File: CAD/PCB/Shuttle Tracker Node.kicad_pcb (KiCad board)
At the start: 2 copper layers, 98.9 x 44.1 mm, 27 parts, among them J1 Conn_01x01, J2 Conn_01x01, J3 Conn_01x01, J4 Conn_01x01, J5 Conn_01x01, J6 Conn_01x01, J7 Conn_01x01, SW1 SW_Push, SW10 SW_Push, SW11 SW_Push, SW12 SW_Push, SW13 PEC11-4215F-S24, SW2 SW_Push, SW3 SW_Push, SW4 SW_Push, SW5 SW_Push, SW6 SW_Push, SW7 SW_Push, SW8 SW_Push, SW9 SW_Push, U1 ESP32-C3-DEVKITC-02

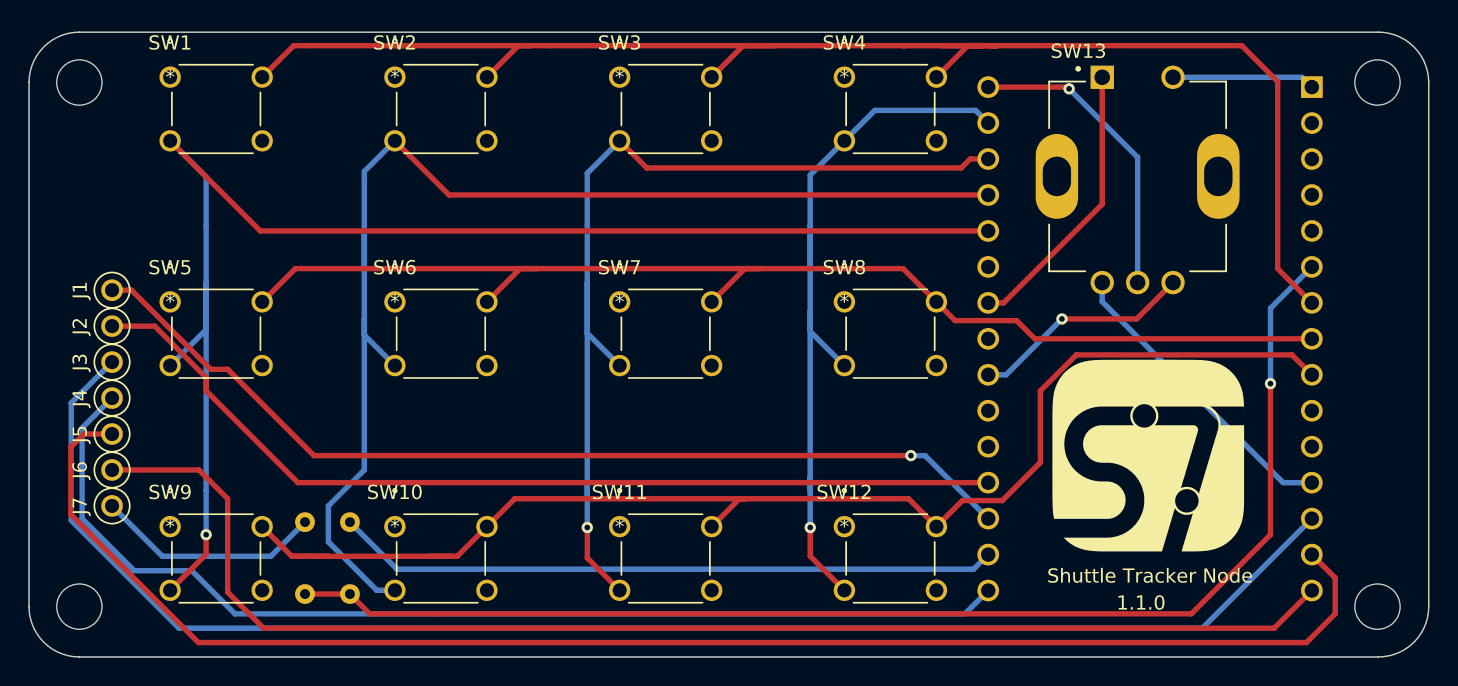
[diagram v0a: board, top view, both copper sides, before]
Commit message: Update fabrication files
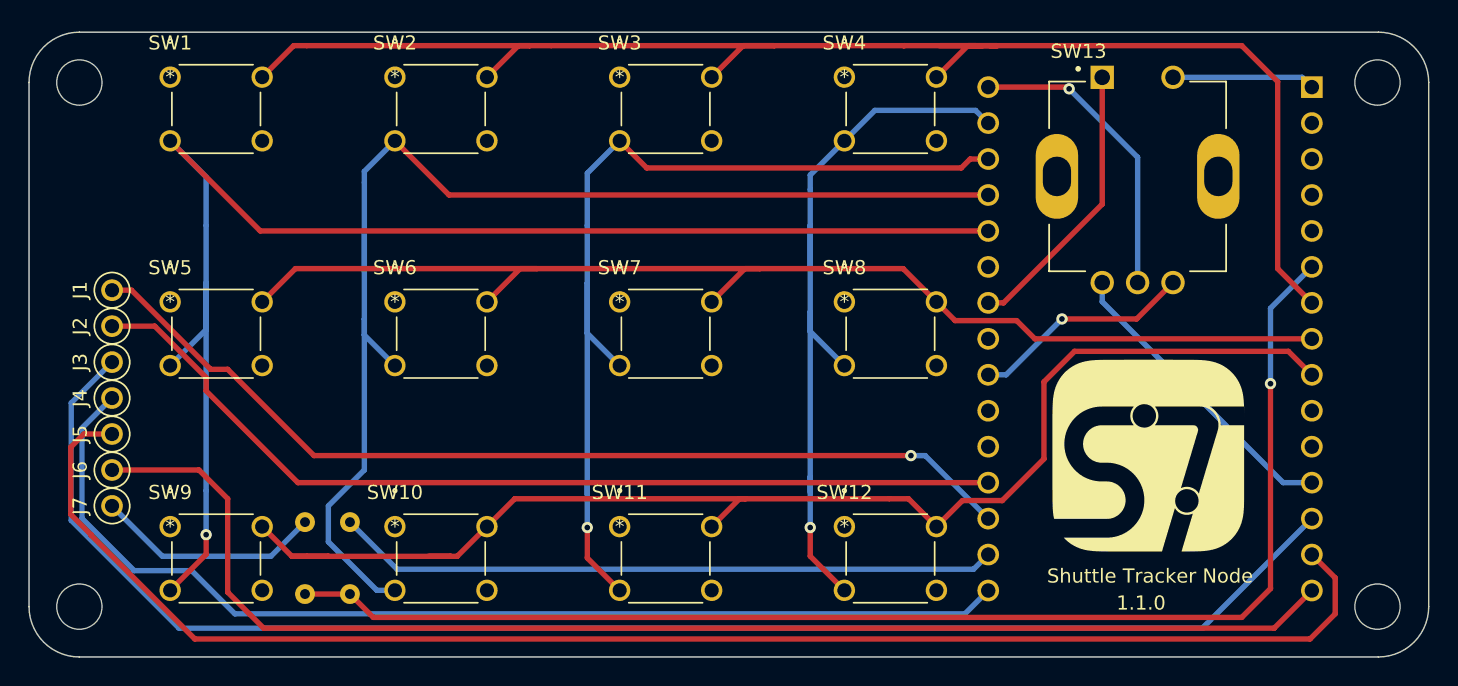
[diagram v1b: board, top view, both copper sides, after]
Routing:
- net V_OUT: track 91.2 -> 93.7 mm
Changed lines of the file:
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@@
       (outputformat 1)
       (mirror false)
-      (drillshape 1)
+      (drillshape 0)
       (scaleselection 1)
-      (outputdirectory "")
+      (outputdirectory "Fabrication/")
     )
   )
@@
   (segment (start 165.608 94.488) (end 181.356 94.488) (width 0.381) (layer "F.Cu") (net 10))
   (segment (start 180.34 110.744) (end 190.5 110.744) (width 0.381) (layer "F.Cu") (net 11))
+  (segment (start 201.422 102.489) (end 203.581 100.33) (width 0.381) (layer "F.Cu") (net 11))
   (segment (start 164.043502 110.744) (end 162.075002 112.7125) (width 0.381) (layer "F.Cu") (net 11))
   (segment (start 146.200002 112.7125) (end 148.295502 114.808) (width 0.381) (layer "F.Cu") (net 11))
   (segment (start 180.34 110.744) (end 164.043502 110.744) (width 0.381) (layer "F.Cu") (net 11))
   (segment (start 159.979502 114.808) (end 162.075002 112.7125) (width 0.381) (layer "F.Cu") (net 11))
-  (segment (start 203.708 100.584) (end 218.9412 100.584) (width 0.381) (layer "F.Cu") (net 11))
   (segment (start 159.512 114.808) (end 159.979502 114.808) (width 0.381) (layer "F.Cu") (net 11))
   (segment (start 195.664347 110.873155) (end 198.477479 110.873155) (width 0.381) (layer "F.Cu") (net 11))
   (segment (start 149.352 114.808) (end 150.876 114.808) (width 0.381) (layer "F.Cu") (net 11))
   (segment (start 148.295502 114.808) (end 150.876 114.808) (width 0.381) (layer "F.Cu") (net 11))
-  (segment (start 201.168 103.124) (end 203.708 100.584) (width 0.381) (layer "F.Cu") (net 11))
-  (segment (start 198.477479 110.873155) (end 201.168 108.182634) (width 0.381) (layer "F.Cu") (net 11))
   (segment (start 148.295502 114.808) (end 149.352 114.808) (width 0.381) (layer "F.Cu") (net 11))
-  (segment (start 201.168 108.182634) (end 201.168 103.124) (width 0.381) (layer "F.Cu") (net 11))
   (segment (start 193.825002 112.7125) (end 191.856502 110.744) (width 0.381) (layer "F.Cu") (net 11))
   (segment (start 179.918502 110.744) (end 180.34 110.744) (width 0.381) (layer "F.Cu") (net 11))
+  (segment (start 218.6872 100.33) (end 220.345 101.9878) (width 0.381) (layer "F.Cu") (net 11))
+  (segment (start 203.581 100.33) (end 218.6872 100.33) (width 0.381) (layer "F.Cu") (net 11))
   (segment (start 157.979501 114.808) (end 159.512 114.808) (width 0.381) (layer "F.Cu") (net 11))
   (segment (start 191.856502 110.744) (end 190.5 110.744) (width 0.381) (layer "F.Cu") (net 11))
+  (segment (start 201.422 107.928634) (end 201.422 102.489) (width 0.381) (layer "F.Cu") (net 11))
   (segment (start 198.477479 110.873155) (end 198.478328 110.874004) (width 0.381) (layer "F.Cu") (net 11))
   (segment (start 177.950002 112.7125) (end 179.918502 110.744) (width 0.381) (layer "F.Cu") (net 11))
   (segment (start 150.876 114.808) (end 159.512 114.808) (width 0.381) (layer "F.Cu") (net 11))
-  (segment (start 218.9412 100.584) (end 220.345 101.9878) (width 0.381) (layer "F.Cu") (net 11))
   (segment (start 193.825002 112.7125) (end 195.664347 110.873155) (width 0.381) (layer "F.Cu") (net 11))
+  (segment (start 198.477479 110.873155) (end 201.422 107.928634) (width 0.381) (layer "F.Cu") (net 11))
   (segment (start 218.3198 109.6078) (end 220.345 109.6078) (width 0.381) (layer "B.Cu") (net 12))
   (segment (start 205.537501 95.475001) (end 205.537501 96.825501) (width 0.381) (layer "B.Cu") (net 12))
@@
   (segment (start 139.150694 114.808) (end 146.812 114.808) (width 0.381) (layer "B.Cu") (net 21))
   (segment (start 146.812 114.808) (end 149.225 112.395) (width 0.381) (layer "B.Cu") (net 21))
-  (segment (start 152.4 117.475) (end 153.797 118.872) (width 0.381) (layer "F.Cu") (net 22))
-  (segment (start 211.836 118.872) (end 217.424 113.284) (width 0.381) (layer "F.Cu") (net 22))
-  (segment (start 158.496 118.872) (end 211.836 118.872) (width 0.381) (layer "F.Cu") (net 22))
-  (segment (start 153.797 118.872) (end 158.496 118.872) (width 0.381) (layer "F.Cu") (net 22))
+  (segment (start 154.051 119.126) (end 215.392 119.126) (width 0.381) (layer "F.Cu") (net 22))
+  (segment (start 215.392 119.126) (end 217.424 117.094) (width 0.381) (layer "F.Cu") (net 22))
   (segment (start 149.225 117.475) (end 152.4 117.475) (width 0.381) (layer "F.Cu") (net 22))
-  (segment (start 217.424 113.284) (end 217.424 102.616) (width 0.381) (layer "F.Cu") (net 22))
+  (segment (start 152.4 117.475) (end 154.051 119.126) (width 0.381) (layer "F.Cu") (net 22))
+  (segment (start 217.424 117.094) (end 217.424 102.616) (width 0.381) (layer "F.Cu") (net 22))
   (via (at 217.424 102.616) (size 0.8) (drill 0.4) (layers "F.Cu" "B.Cu") (net 22))
   (segment (start 217.424 97.2888) (end 220.345 94.3678) (width 0.381) (layer "B.Cu") (net 22))
@@
   (segment (start 208.037501 95.475001) (end 208.037501 86.625501) (width 0.381) (layer "B.Cu") (net 28))
   (segment (start 208.037501 86.625501) (end 203.2 81.788) (width 0.381) (layer "B.Cu") (net 28))
-  (segment (start 141.696565 120.904) (end 134.112 113.319435) (width 0.381) (layer "F.Cu") (net 29))
-  (segment (start 219.964 120.904) (end 141.696565 120.904) (width 0.381) (layer "F.Cu") (net 29))
-  (segment (start 134.112 113.284) (end 132.684681 111.856681) (width 0.381) (layer "F.Cu") (net 29))
-  (segment (start 134.112 113.319435) (end 134.112 113.284) (width 0.381) (layer "F.Cu") (net 29))
   (segment (start 221.996 116.3388) (end 221.996 118.872) (width 0.381) (layer "F.Cu") (net 29))
-  (segment (start 221.996 118.872) (end 219.964 120.904) (width 0.381) (layer "F.Cu") (net 29))
   (segment (start 220.345 114.6878) (end 221.996 116.3388) (width 0.381) (layer "F.Cu") (net 29))
   (segment (start 132.684681 111.856681) (end 132.684681 107.091319) (width 0.381) (layer "F.Cu") (net 29))
+  (segment (start 133.604 106.172) (end 135.594694 106.172) (width 0.381) (layer "F.Cu") (net 29))
   (segment (start 132.684681 107.091319) (end 133.604 106.172) (width 0.381) (layer "F.Cu") (net 29))
-  (segment (start 133.604 106.172) (end 135.594694 106.172) (width 0.381) (layer "F.Cu") (net 29))
+  (segment (start 141.442565 120.65) (end 134.112 113.319435) (width 0.381) (layer "F.Cu") (net 29))
+  (segment (start 134.112 113.319435) (end 134.112 113.284) (width 0.381) (layer "F.Cu") (net 29))
+  (segment (start 220.218 120.65) (end 141.442565 120.65) (width 0.381) (layer "F.Cu") (net 29))
+  (segment (start 134.112 113.284) (end 132.684681 111.856681) (width 0.381) (layer "F.Cu") (net 29))
+  (segment (start 221.996 118.872) (end 220.218 120.65) (width 0.381) (layer "F.Cu") (net 29))
   (segment (start 220.345 117.2278) (end 217.6848 119.888) (width 0.381) (layer "F.Cu") (net 30))
   (segment (start 143.764 110.744) (end 141.732 108.712) (width 0.381) (layer "F.Cu") (net 30))
